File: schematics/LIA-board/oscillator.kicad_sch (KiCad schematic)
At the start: 7 parts, among them U6 OPA2196xD

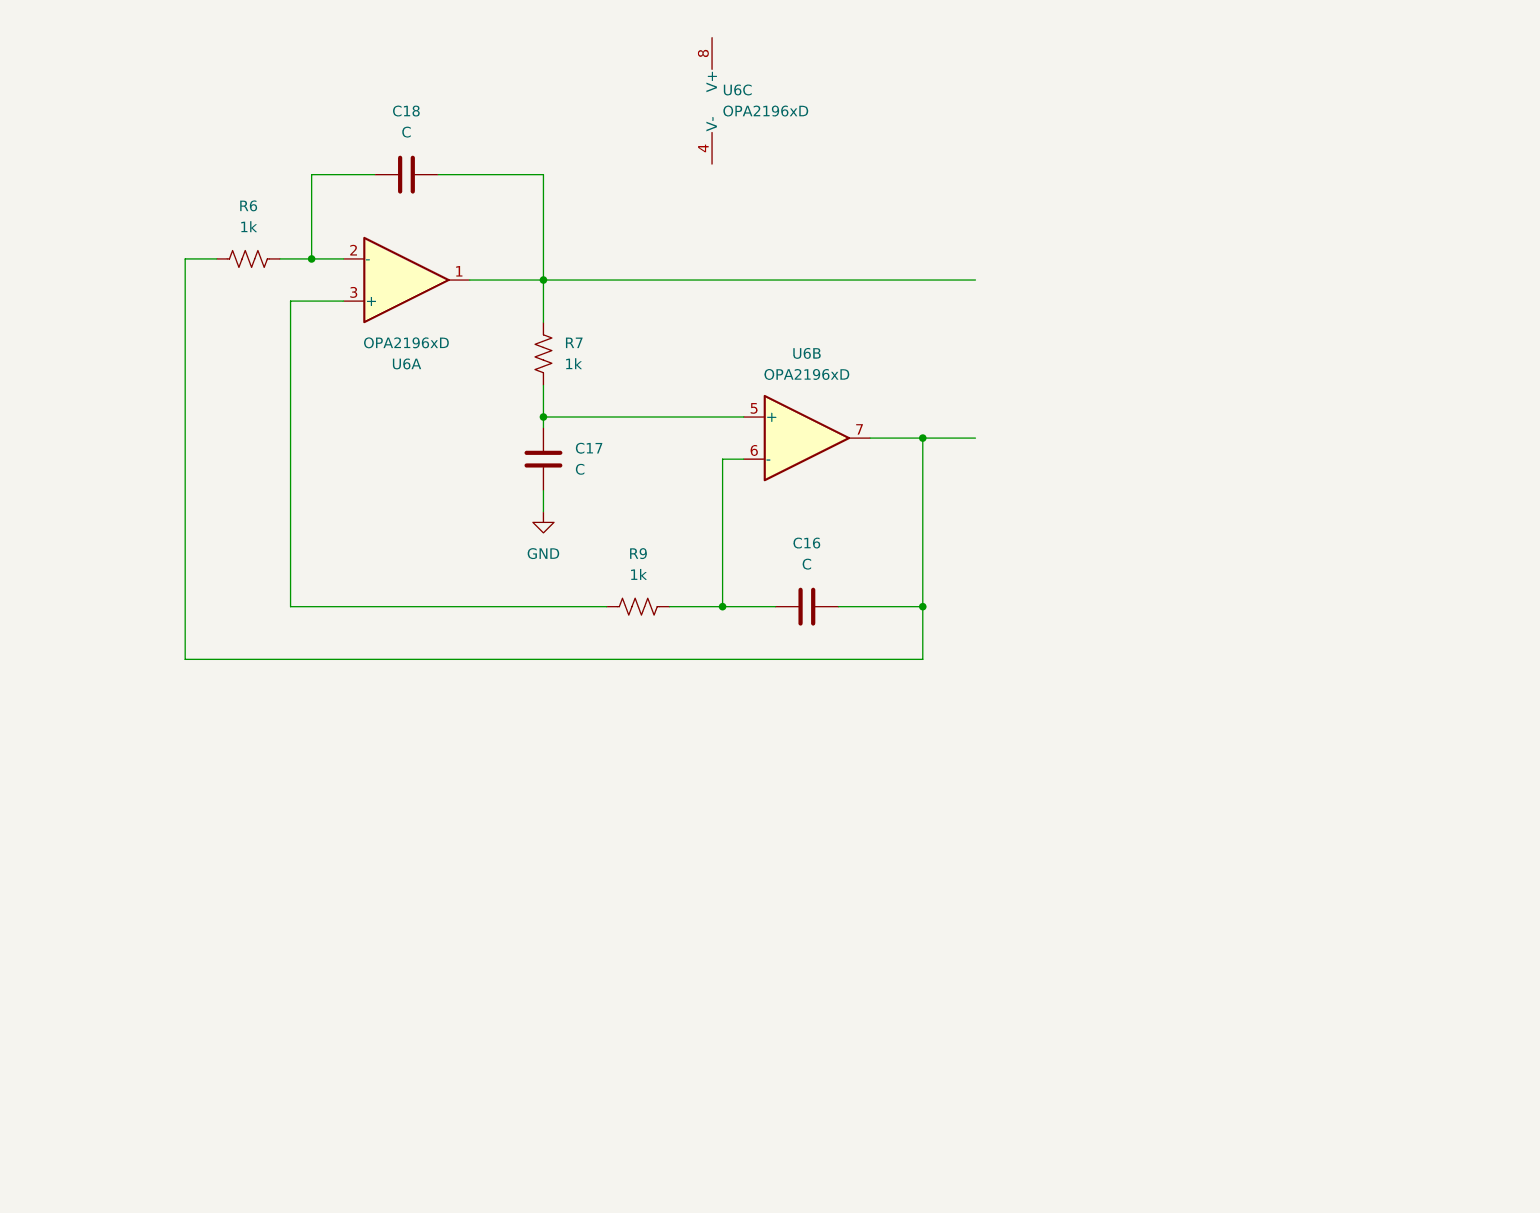
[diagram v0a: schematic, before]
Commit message: additions to pcb
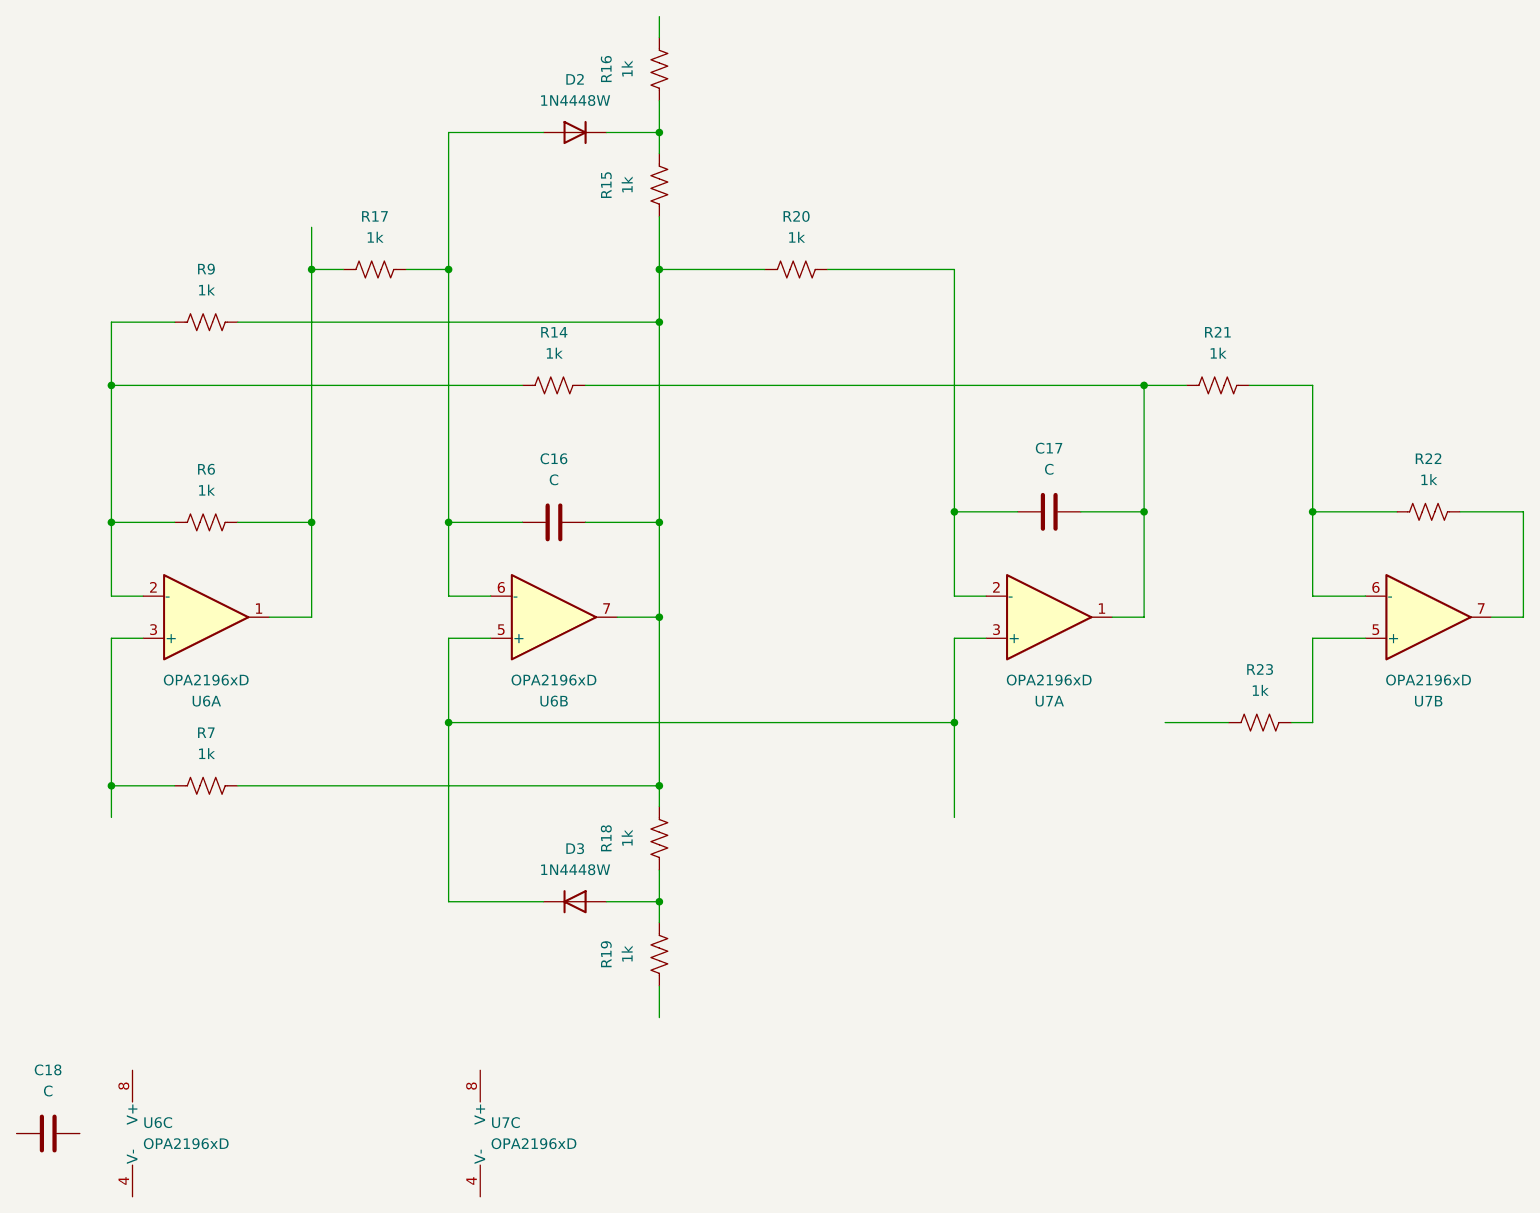
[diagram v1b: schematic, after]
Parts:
- added D2, D3: 1N4448W, Diode_SMD:D_SOD-123, symbol Diode:1N4448W
- added R14, R15, R16, R17, R18, R19, R20, R21, R22, R23: 1k, SparkFun-Resistor:R_0603_1608Metric, symbol SparkFun:R
- added U7: OPA2196xD, Package_SO:SOIC-8_3.9x4.9mm_P1.27mm, symbol Amplifier_Operational:OPA2196xD
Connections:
- net at C16.2, U6.7: now also R7.2, R9.1, R15.2, R18.1, R20.2; no longer R6.2
- net at C16.1, U6.6 (-): now also D2.2 (A), R17.1; no longer R9.1
- net at R9.2: now also R6.2, U6.2 (-), R14.2; no longer U6.3 (+)
- net GND: no longer names the net of C17.2
- net GND: now also R14.1, R21.2, U7.1
- new net: R17.2, R6.1, U6.1
- new net: D2.1 (K), R15.1, R16.2
- new net: R7.1, U6.3 (+)
- new net: C17.1, R20.1, U7.2 (-)
- new net: D3.1 (K), U6.5 (+), U7.3 (+)
- new net: R23.1, U7.5 (+)
- new net: R21.1, R22.2, U7.6 (-)
- new net: R22.1, U7.7
- new net: D3.2 (A), R18.2, R19.1
- now unconnected: C18.1, C18.2
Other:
- moved on the sheet: C16, C17, C18, R6, R7, R9, U6A, U6B, U6C
